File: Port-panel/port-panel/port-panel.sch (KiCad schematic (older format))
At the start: 4 parts

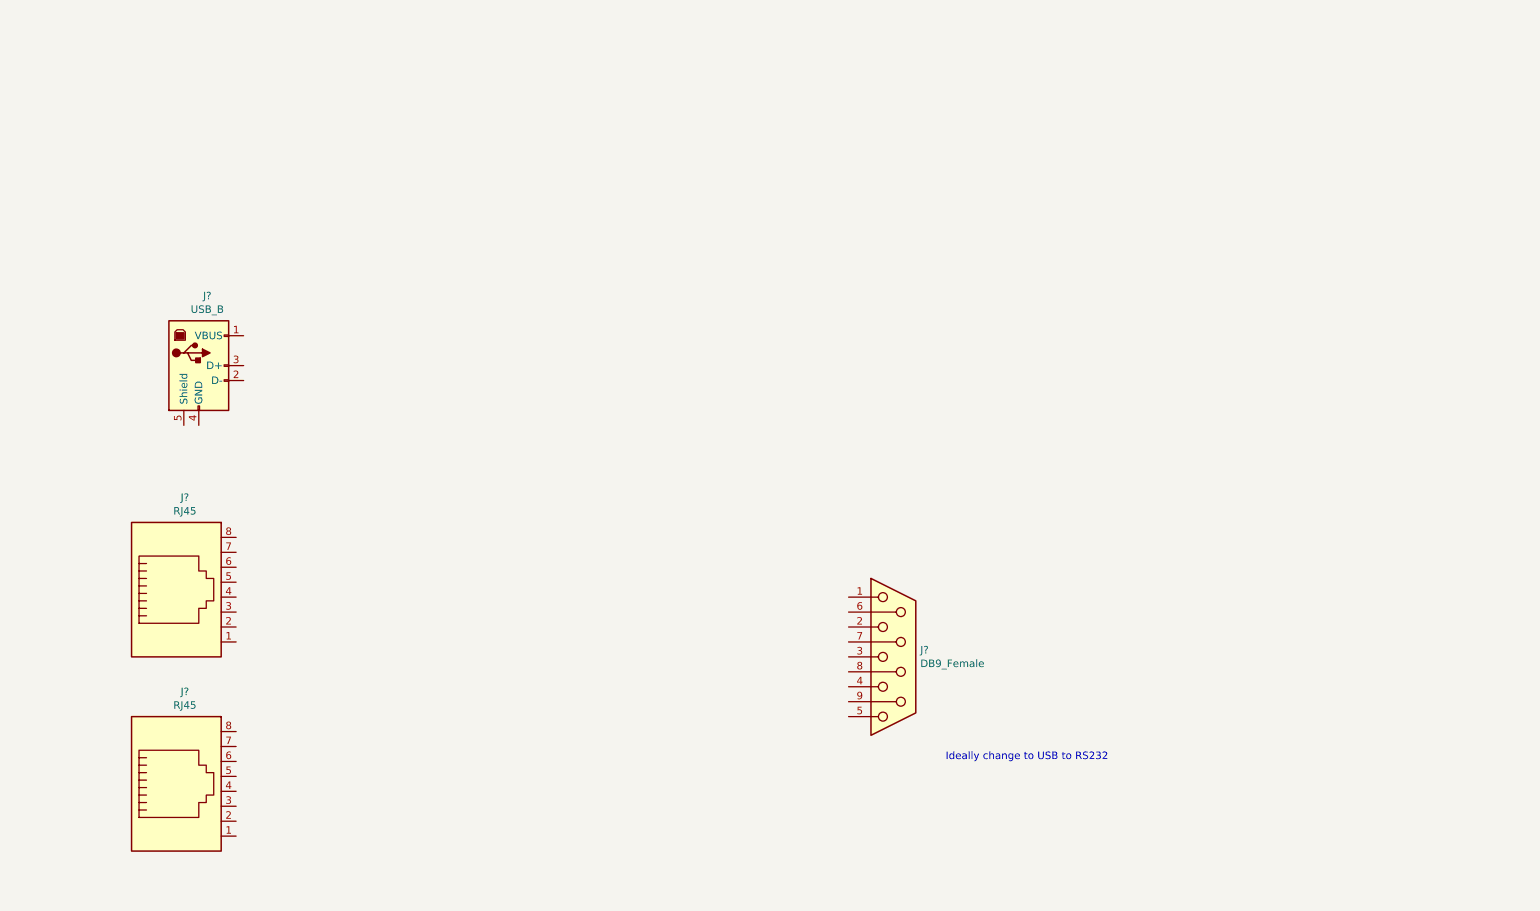
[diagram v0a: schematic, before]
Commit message: Work on port panel
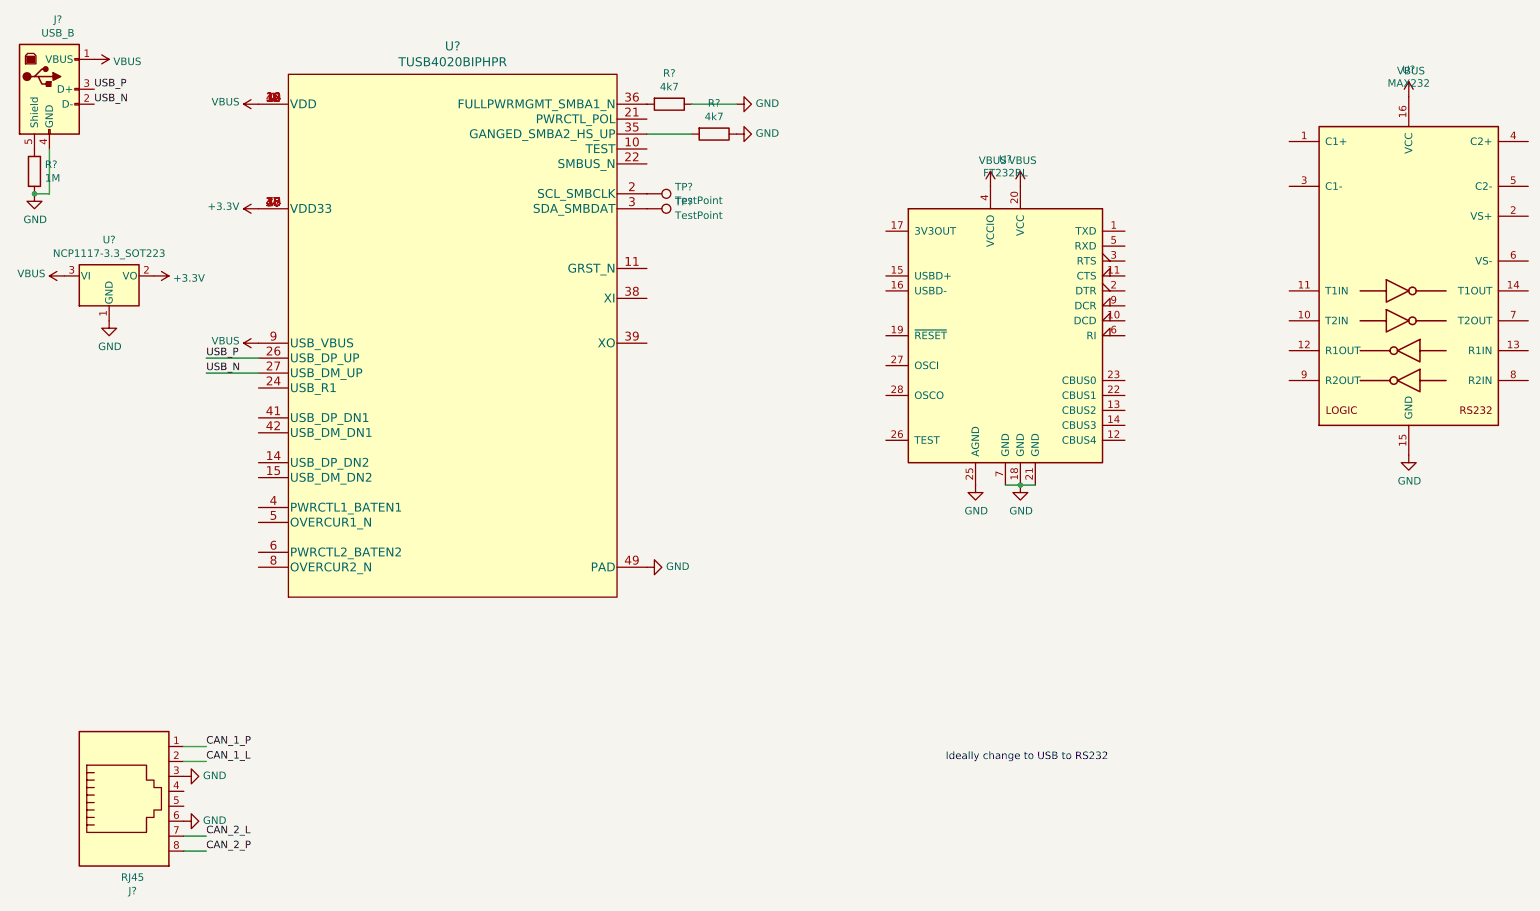
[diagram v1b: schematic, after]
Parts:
- removed J?: RJ45, symbol Connector:RJ45
- removed J?: DB9_Female, symbol Connector:DB9_Female
- added R?: 1M, symbol Device:R
- added R? (x2): 4k7, symbol Device:R
- added TP? (x2): TestPoint, symbol Connector:TestPoint
- added U?: FT232RL, Package_SO:SSOP-28_5.3x10.2mm_P0.65mm, symbol Interface_USB:FT232RL
- added U?: MAX232, symbol Interface_UART:MAX232
- added U?: TUSB4020BIPHPR, PHP0048E_N, symbol AERO_custom_symbols:TUSB4020BIPHPR
- added U?: NCP1117-3.3_SOT223, Package_TO_SOT_SMD:SOT-223-3_TabPin2, symbol Regulator_Linear:NCP1117-3.3_SOT223
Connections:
- net VBUS: now reaches J?.1 (VBUS)
- net VBUS: now also U?.1 (VDD), U?.12 (VDD), U?.16 (VCC), U?.18 (VDD), U?.20 (VCC), U?.3 (VI), U?.30 (VDD), U?.34 (VDD), U?.4 (VCCIO), U?.45 (VDD), U?.9 (USB_VBUS)
- net USB_N: now reaches J?.2 (D-)
- net USB_N: now also U?.27 (USB_DM_UP)
- net USB_P: now reaches J?.3 (D+)
- net USB_P: now also U?.26 (USB_DP_UP)
- net GND: now reaches J?.4 (GND)
- net GND: now also J?.3, J?.6, R?.1, R?.1, R?.2, U?.1 (GND), U?.15 (GND), U?.18 (GND), U?.21 (GND), U?.25 (AGND), U?.49 (PAD), U?.7 (GND)
- net at J?.5 (Shield): now also R?.1
- net CAN_1_P: now reaches J?.1
- net CAN_1_L: now reaches J?.2
- net CAN_2_L: now reaches J?.7
- net CAN_2_P: now reaches J?.8
- new net: TP?.1, U?.2 (SCL_SMBCLK)
- new net: TP?.1, U?.3 (SDA_SMBDAT)
- new net: R?.2, U?.35 (GANGED_SMBA2_HS_UP)
- new net: R?.2, U?.36 (FULLPWRMGMT_SMBA1_N)
- new net +3V3: U?.13 (VDD33), U?.2 (VO), U?.23 (VDD33), U?.25 (VDD33), U?.33 (VDD33), U?.37 (VDD33), U?.40 (VDD33), U?.48 (VDD33), U?.7 (VDD33)
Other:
- moved on the sheet: J?
